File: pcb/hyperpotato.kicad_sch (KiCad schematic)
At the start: 60 parts, among them J2 Conn_01x02_Socket, J3 Conn_01x04, J4 Conn_01x04, J5 Conn_01x04, J6 Conn_01x12_Socket, J7 Conn_01x12_Socket, K1 SW_Push, K10 SW_Push, K11 SW_Push, K12 SW_Push, K13 SW_Push, K14 SW_Push, K15 SW_Push, K16 SW_Push, K17 SW_Push, K2 SW_Push, K3 SW_Push, K4 SW_Push, K5 SW_Push, K6 SW_Push, K7 SW_Push, K8 SW_Push, K9 SW_Push, SW1 SW_Push, SW2 SW_SPDT, U1 ProMicro

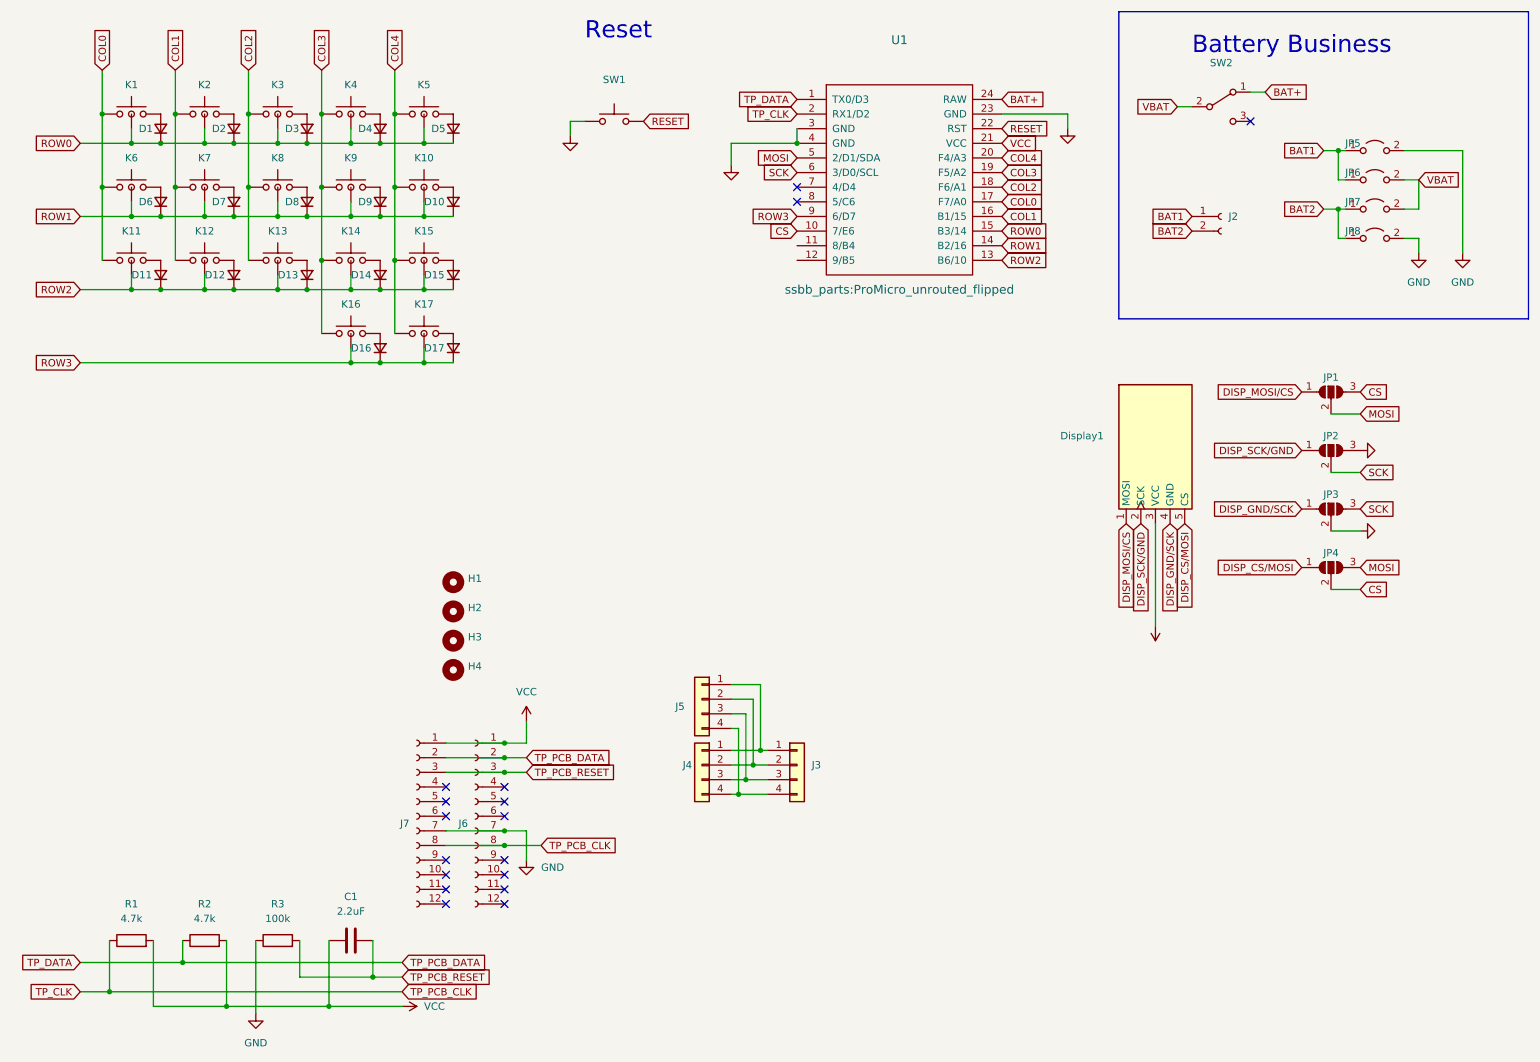
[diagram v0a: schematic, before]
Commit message: Prepare rev1.3
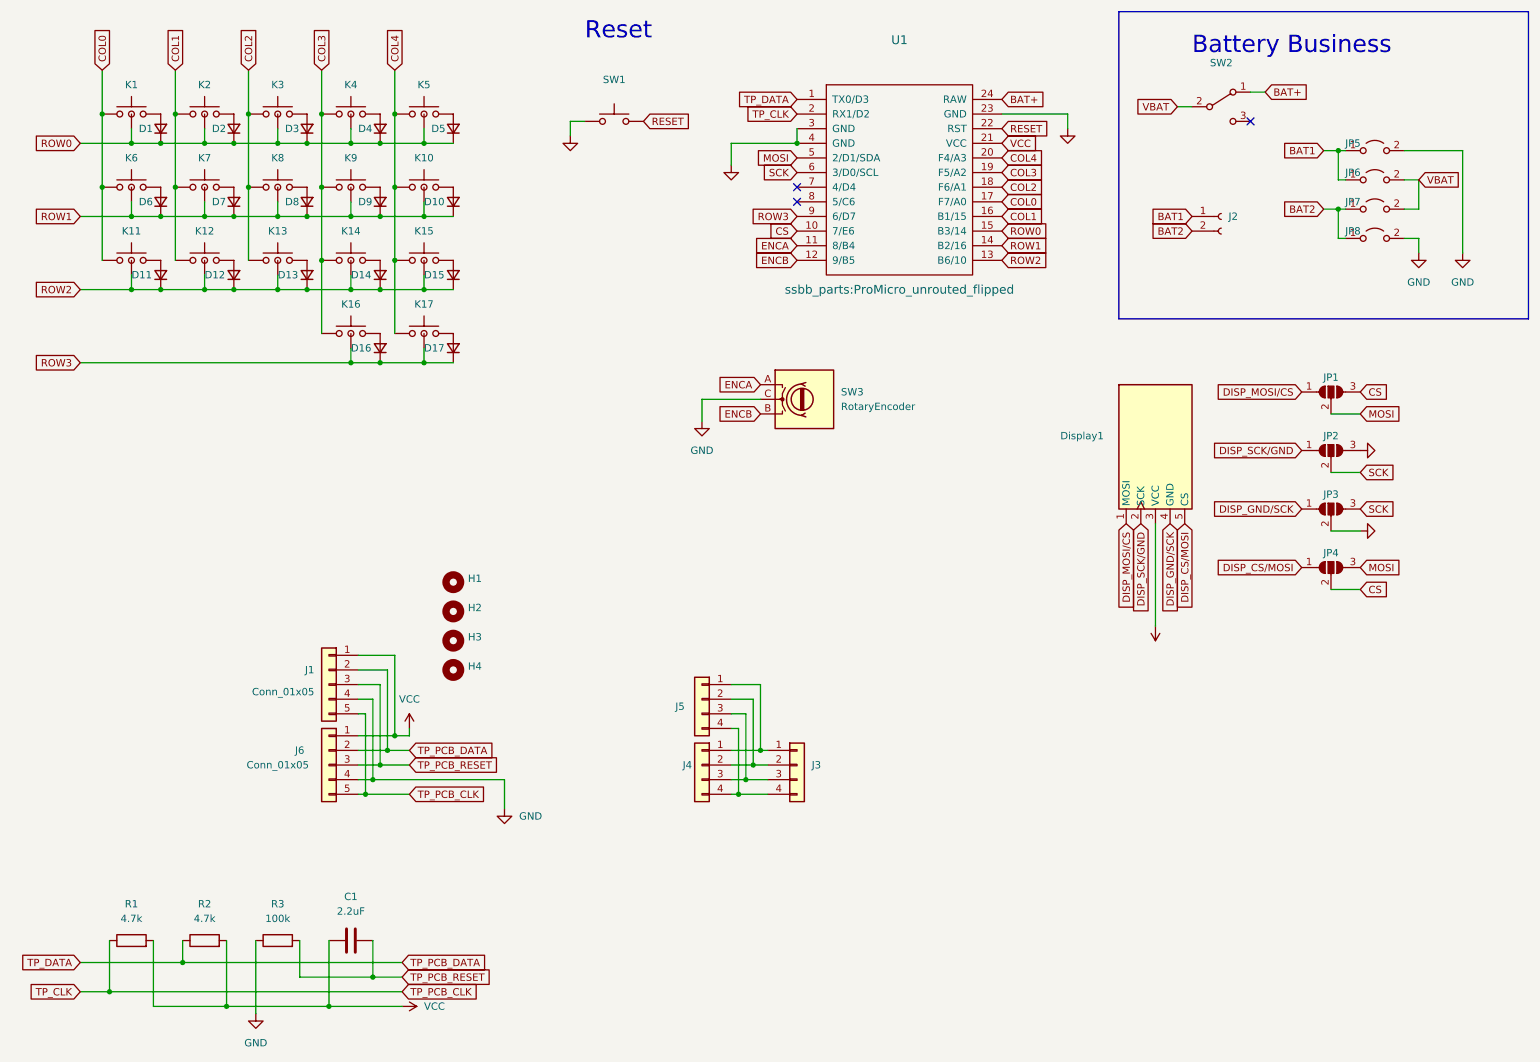
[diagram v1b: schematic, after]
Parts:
- removed J6, J7: Conn_01x12_Socket, hyperpotato:Trackpoint_PCB_Connector, symbol Connector:Conn_01x12_Socket
- added J1, J6: Conn_01x05, hyperpotato:Trackpoint_PCB_Connector_alt, symbol Connector_Generic:Conn_01x05
- added SW3: RotaryEncoder, hyperpotato:RotaryEncoder_Alps_EC12E_Vertical_H20mm, symbol Device:RotaryEncoder
- K17: footprint hyperpotato:V1_V2_HS_reversible_plated_no_fix_pin -> hyperpotato:V1_V2_HS_reversible_plated
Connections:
- net GND: now also J1.4 (Pin_4), J6.4 (Pin_4), SW3.C
- net TP_CLK: now also J1.5 (Pin_5), J6.5 (Pin_5)
- net TP_DATA: now also J1.2 (Pin_2), J6.2 (Pin_2)
- net TP_PCB_RESET: now also J1.3 (Pin_3), J6.3 (Pin_3)
- net VCC: now also J1.1 (Pin_1), J6.1 (Pin_1)
- net ENCA: now reaches U1.11 (8/B4)
- net ENCA: now also SW3.A
- net ENCB: now reaches U1.12 (9/B5)
- net ENCB: now also SW3.B
- no-connect marks 17 -> 3
